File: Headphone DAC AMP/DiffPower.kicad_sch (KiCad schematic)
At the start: 11 parts, among them U6 MCP1727-1802xSN, U7 MCP1727-3302xSN, U9 TPS717XX

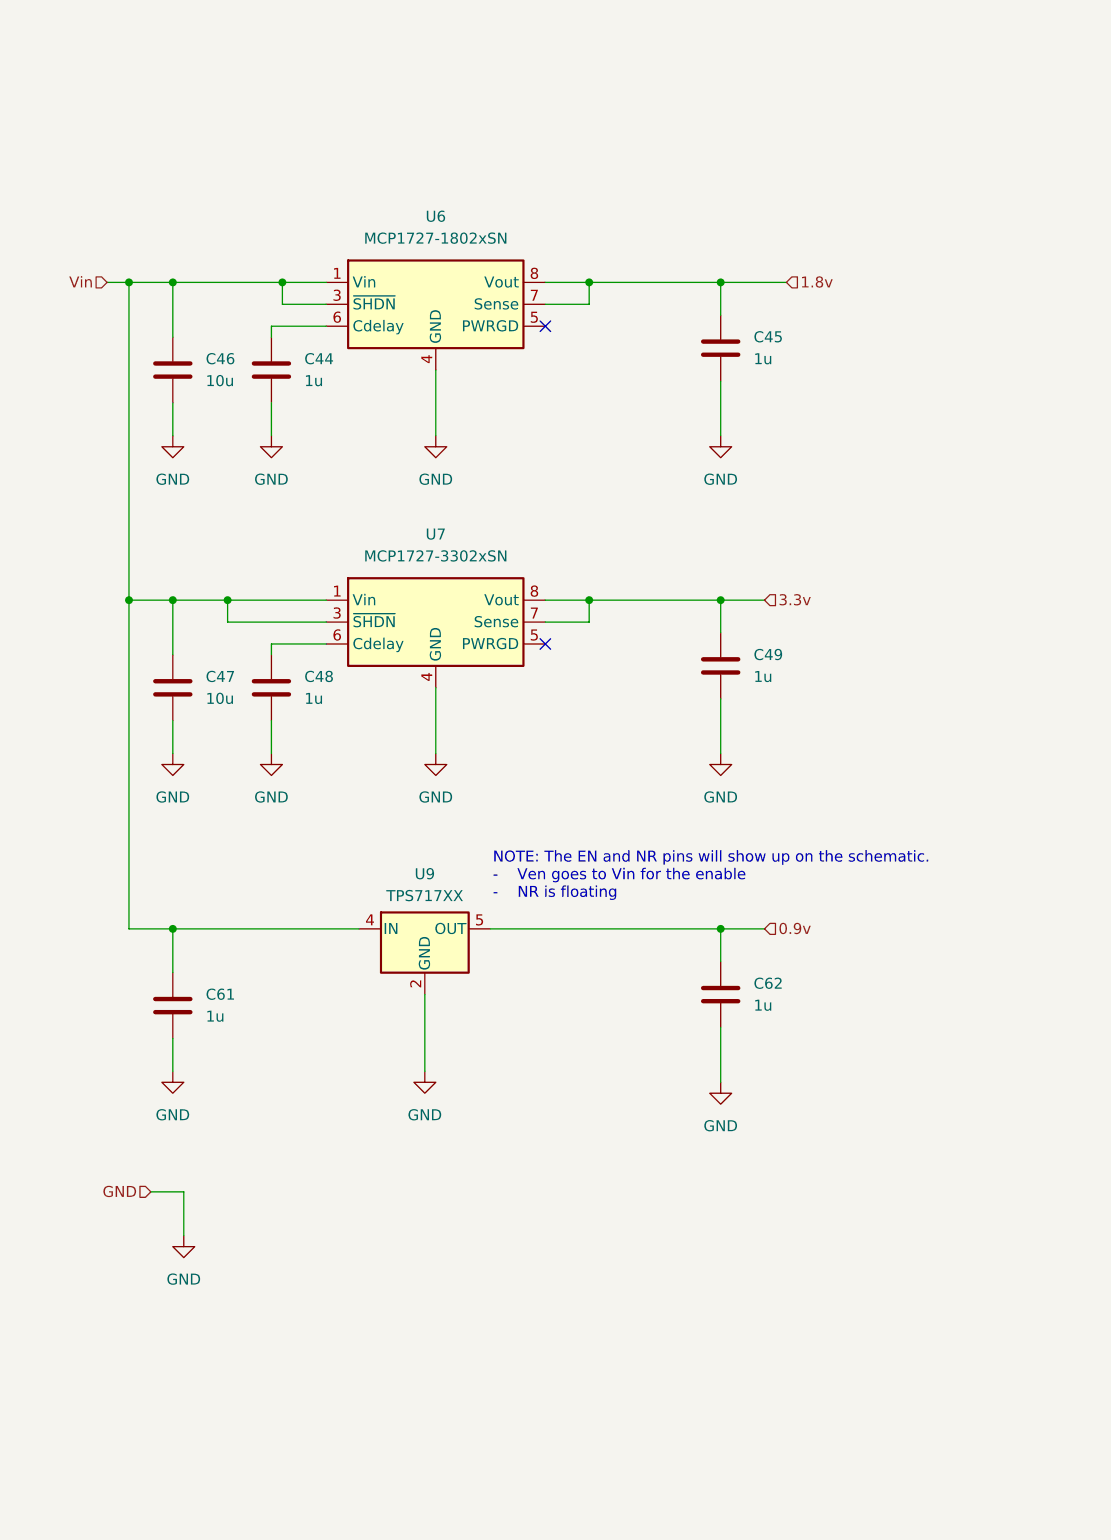
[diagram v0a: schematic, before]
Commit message: Cleaned up shcematic more
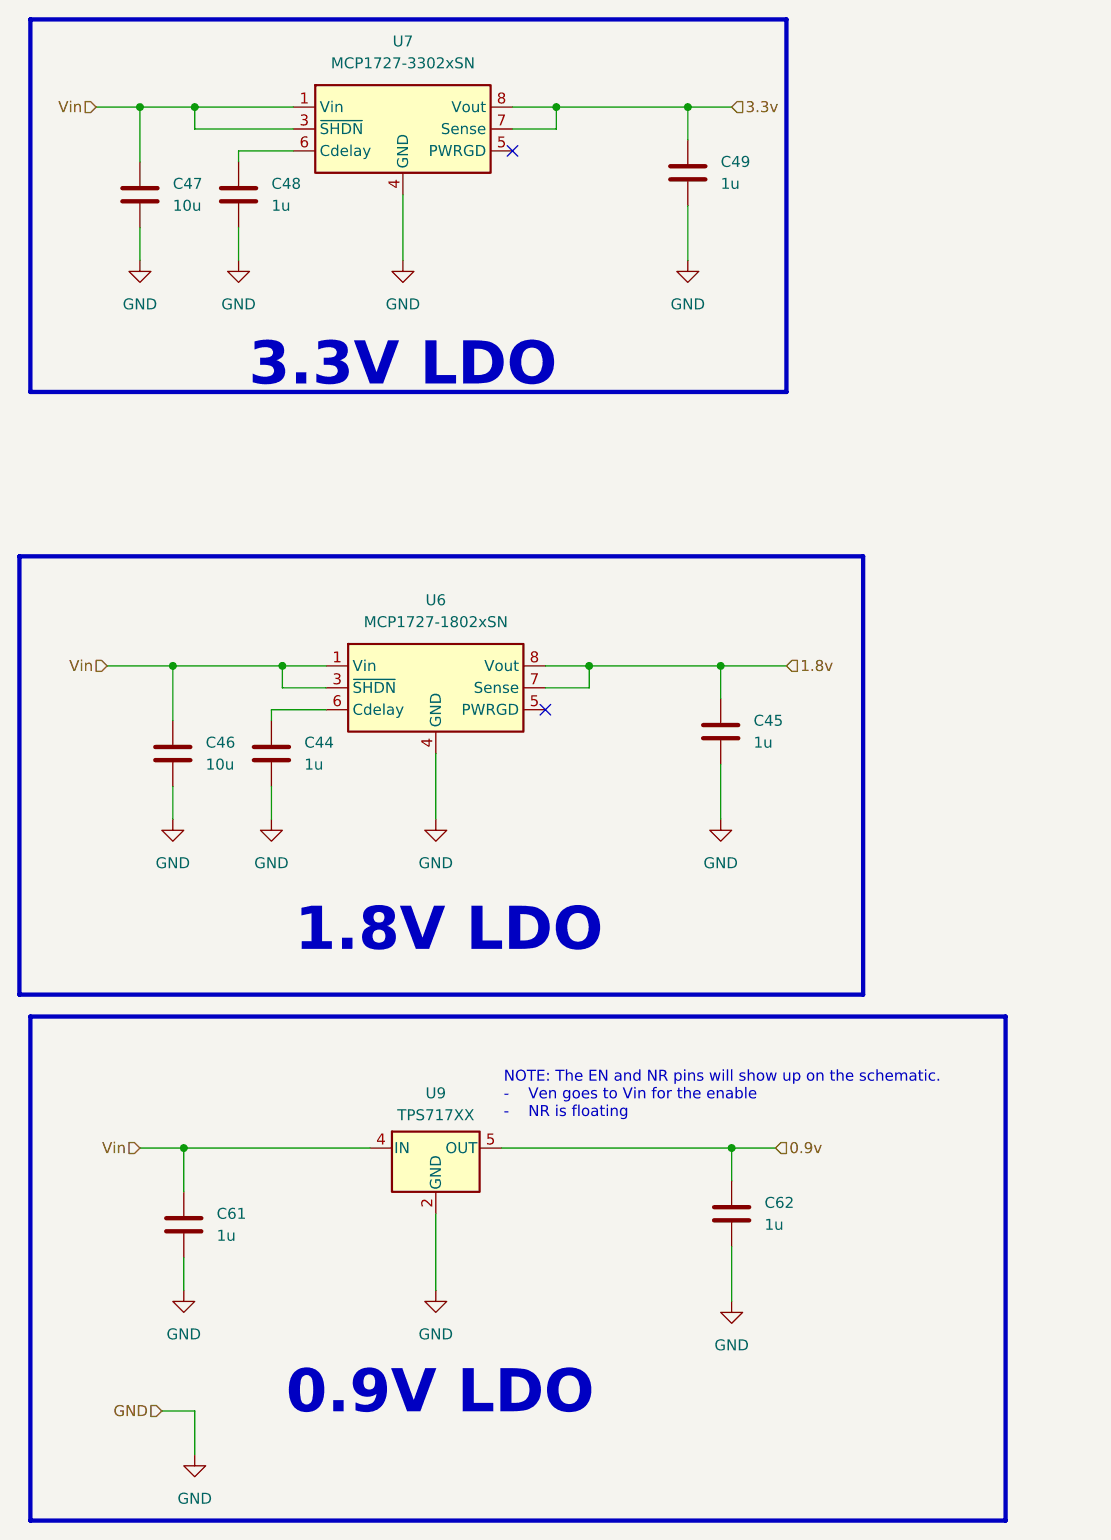
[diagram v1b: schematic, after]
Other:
- note added: "0.9V LDO"
- note added: "1.8V LDO"
- note added: "3.3V LDO"
- moved on the sheet: C44, C45, C46, C47, C48, C49, C61, C62, U6, U7, U9
